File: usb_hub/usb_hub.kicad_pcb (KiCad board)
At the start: 2 copper layers, 100 x 23 mm, 120 parts, among them P1 CONN_01X02, U1 TPS2044B, U10 USB_A_FEMALE, U11 SN75240, U12 SN75240, U13 USB_A_FEMALE, U14 USB_A_FEMALE, U15 USB_A_FEMALE, U16 USB_A_FEMALE, U2 TPS2044B, U3 TUSB2077A, U4 TPS76333, U5 USB_A_MALE, U6 SN75240, U7 SN75240, U8 USB_A_FEMALE, U9 USB_A_FEMALE, X1 6 MHz

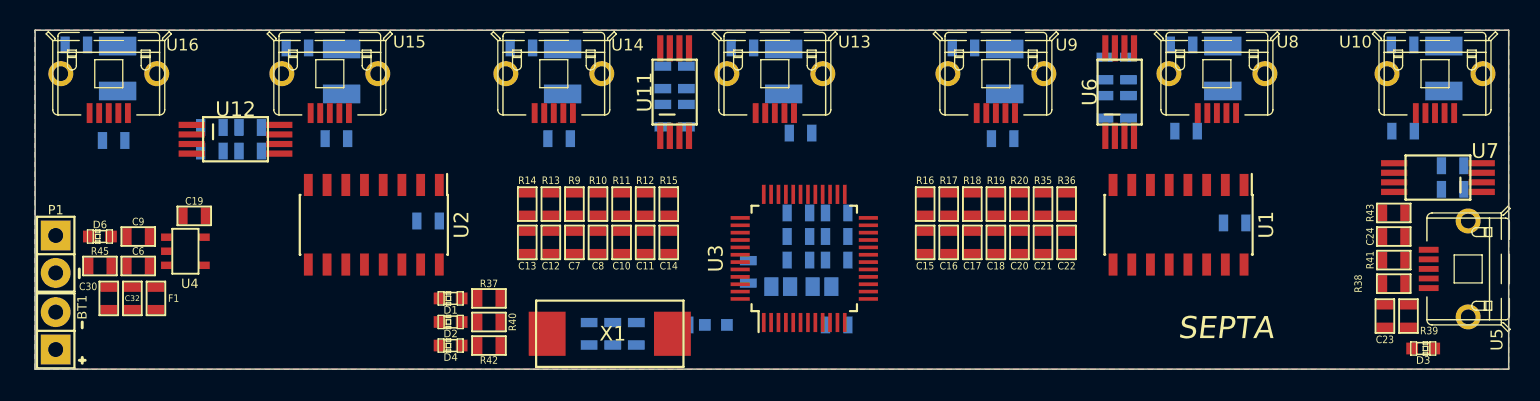
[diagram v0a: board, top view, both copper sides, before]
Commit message: finished routing. need to check bom and trace widths and pos file
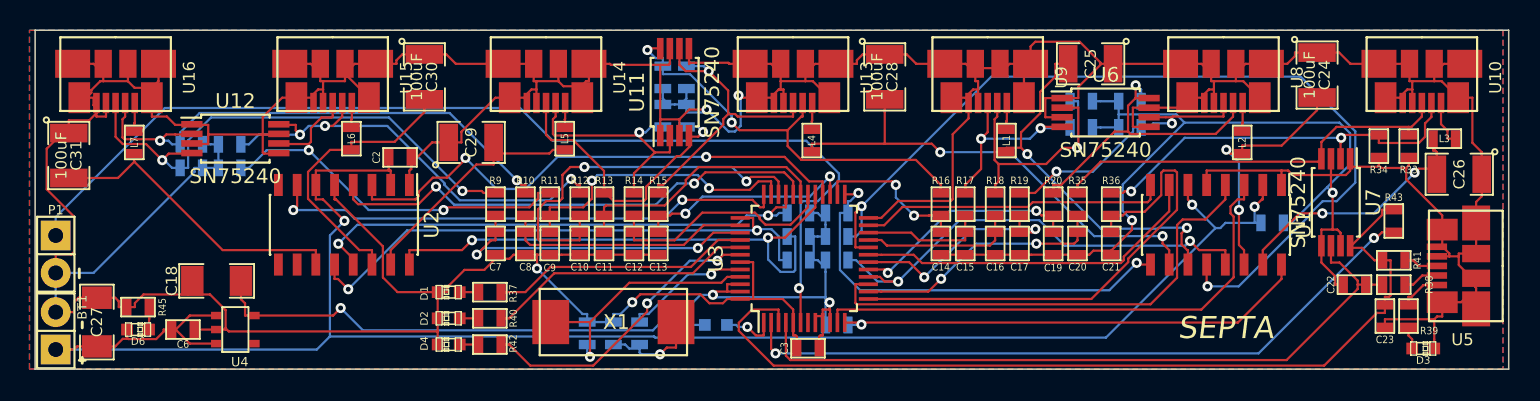
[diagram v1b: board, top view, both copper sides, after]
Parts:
- removed C32: 4.7uF, SMD_Packages:SMD-0603
- removed C33, C34, C35, C36: 100uF, SMD_Packages:SMD-1210
- removed C37, C38, C39, C40: .1uF, SMD_Packages:SMD-0603
- removed F1: FUSE, SMD_Packages:SMD-0603
- removed JP1, JP2: JUMPER, Connect:GS2
- C18: value 22pF -> 10uF; footprint SMD_Packages:SMD-0603 -> SMD_Packages:SMD-1206
- C19: value 4.7uF -> 22pF
- C2, C25, C26, C29, C3, L1, L2, L3, L4, L5, L6, L7, R33, R34: moved to F.Cu
- C24: value 22pF -> 100uF; footprint SMD_Packages:SMD-0603 -> SMD_Packages:SMD-1210
- C27: value .1uF -> 10uF; footprint SMD_Packages:SMD-0603 -> SMD_Packages:SMD-1206; moved to F.Cu
- C28, C31: value .1uF -> 100uF; footprint SMD_Packages:SMD-0603 -> SMD_Packages:SMD-1210; moved to F.Cu
- C30: value .1uF -> 100uF; footprint SMD_Packages:SMD-0603 -> SMD_Packages:SMD-1210
- C6: value 4.7uF -> 1uF
- C9: value .1uF -> 22pF
- D1, D2, D4, D6: value LED(G) -> LED
- R10, R11, R12, R13, R14, R15, R16, R17, R18, R19, R20, R35, R36, R38, R41, R9: value 27 -> 30
- R37, R39, R40, R42, R44, R45: value 510 -> 1k
- U10, U13, U14, U15, U16, U8, U9: value USB_A_FEMALE -> USB_MICRO_OUT; footprint ab2_usb:AB2_USB_MICRO_SMD -> apro_lib:MICRO_USB
- U11, U12, U6, U7: footprint usb_hub:TSSOP8 -> Housings_SSOP:TSSOP-8_4.4x3mm_Pitch0.65mm
- U5: footprint ab2_usb:AB2_USB_MICRO_SMD -> apro_lib:MICRO_USB
- moved C31 90.8 mm to (137.3, 87.5), turned to 270 degrees
- moved C27 76.0 mm to (139.2, 98.8), turned to 90 degrees
- moved C29 66.2 mm to (164.6, 86.6), turned to 0 degrees
- moved C19 58.3 mm to (204.1, 93.5), turned to 270 degrees
- moved C18 52.9 mm to (147.3, 96.0), turned to 180 degrees
- moved C26 31.6 mm to (231.6, 88.8), turned to 180 degrees
- moved C9 27.9 mm to (169.9, 93.5), turned to 270 degrees
- moved C30 26.2 mm to (161.4, 82.2), turned to 270 degrees
- moved C22 19.7 mm to (224.5, 96.3), turned to 180 degrees
- moved C14 18.5 mm to (196.5, 93.5)
- moved C24 12.1 mm to (222.0, 82.0), turned to 270 degrees
- moved C25 8.98 mm to (206.6, 81.3), turned to 180 degrees
- moved C13 8.89 mm to (177.3, 93.5)
- moved R14 7.24 mm to (175.6, 90.8)
- moved U7 7.13 mm to (223.3, 90.7), turned to 270 degrees
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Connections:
- BT1 pad 1: Net-(BT1-Pad1) -> VCC
- C18 pad 1: Net-(C18-Pad1) -> 3.3V
- C19 pad 1: 3.3V -> Net-(C19-Pad1)
- C22 pad 1: Net-(C22-Pad1) -> DM0
- C23 pad 1: DM0 -> DP0
- C24 pad 1: DP0 -> GND
- C24 pad 2: GND -> OUT2
- C25 pad 2: OUT2 -> OUT3
- C26 pad 2: OUT3 -> OUT1
- C27 pad 1: GND -> VCC
- C27 pad 2: OUT2 -> GND
- C28 pad 2: OUT3 -> OUT4
- C29 pad 2: OUT1 -> OUT5
- C30 pad 1: Net-(BT1-Pad1) -> GND
- C30 pad 2: GND -> OUT6
- C31 pad 2: OUT1 -> OUT7
- C9 pad 1: VCC -> Net-(C9-Pad1)
- R11 pad 1: Net-(C10-Pad1) -> Net-(C9-Pad1)
- R12 pad 1: Net-(C11-Pad1) -> Net-(C10-Pad1)
- R13 pad 1: Net-(C12-Pad1) -> Net-(C11-Pad1)
- R14 pad 1: Net-(C13-Pad1) -> Net-(C12-Pad1)
- R15 pad 1: Net-(C14-Pad1) -> Net-(C13-Pad1)
- R16 pad 1: Net-(C15-Pad1) -> Net-(C14-Pad1)
- R17 pad 1: Net-(C16-Pad1) -> Net-(C15-Pad1)
- R18 pad 1: Net-(C17-Pad1) -> Net-(C16-Pad1)
- R19 pad 1: Net-(C18-Pad1) -> Net-(C17-Pad1)
- R20 pad 1: Net-(C20-Pad1) -> Net-(C19-Pad1)
- R35 pad 1: Net-(C21-Pad1) -> Net-(C20-Pad1)
- R36 pad 1: Net-(C22-Pad1) -> Net-(C21-Pad1)
- R38 pad 1: Net-(R38-Pad1) -> DM0
- R38 pad 2: DM0 -> Net-(R38-Pad2)
- R41 pad 1: Net-(R41-Pad1) -> DP0
- R41 pad 2: DP0 -> Net-(R41-Pad2)
- R43 pad 1: DP0 -> DP0PUR
- R43 pad 2: DP0PUR -> DP0
- U3 pad 13: Net-(C22-Pad1) -> Net-(C21-Pad1)
- U3 pad 14: Net-(C21-Pad1) -> Net-(C20-Pad1)
- U3 pad 17: Net-(C20-Pad1) -> Net-(C19-Pad1)
- U3 pad 18: Net-(C18-Pad1) -> Net-(C17-Pad1)
- U3 pad 21: Net-(C17-Pad1) -> Net-(C16-Pad1)
- U3 pad 22: Net-(C16-Pad1) -> Net-(C15-Pad1)
- U3 pad 26: Net-(C15-Pad1) -> Net-(C14-Pad1)
- U3 pad 27: Net-(C14-Pad1) -> Net-(C13-Pad1)
- U3 pad 30: Net-(C13-Pad1) -> Net-(C12-Pad1)
- U3 pad 31: Net-(C12-Pad1) -> Net-(C11-Pad1)
- U3 pad 34: Net-(C11-Pad1) -> Net-(C10-Pad1)
- U3 pad 35: Net-(C10-Pad1) -> Net-(C9-Pad1)
- U3 pad 8: Net-(JP1-Pad2) -> 3.3V
- U5 pad 2: Net-(R38-Pad1) -> Net-(R38-Pad2)
- U5 pad 3: Net-(R41-Pad1) -> Net-(R41-Pad2)
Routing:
- net GND: track 0.00 -> 481.1 mm, vias 0 -> 6
- net VCC: track 0.00 -> 127.5 mm, vias 0 -> 3
- net RST: track 0.00 -> 71.2 mm, vias 0 -> 1
- net 3.3V: track 0.00 -> 64.3 mm, vias 0 -> 3
- net OC3: track 0.00 -> 63.3 mm, vias 0 -> 2
- net DP0: track 0.00 -> 62.1 mm
- net DM0: track 0.00 -> 48.9 mm
- net DP0PUR: track 0.00 -> 47.6 mm, vias 0 -> 2
- net OC7: track 0.00 -> 37.3 mm, vias 0 -> 2
- net OC5: track 0.00 -> 37.2 mm, vias 0 -> 2
- net PWRON5: track 0.00 -> 36.3 mm, vias 0 -> 2
- net DM7: track 0.00 -> 36.2 mm, vias 0 -> 2
- net DP7: track 0.00 -> 35.8 mm, vias 0 -> 2
- net PWRON1: track 0.00 -> 35.7 mm
- net PWRON7: track 0.00 -> 35.6 mm, vias 0 -> 2
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- added copper zone on B.Cu, net (none)
- added copper zone on F.Cu, net (none)
- removed copper zone on B.Cu, net GND
- removed copper zone on F.Cu, net GND
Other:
- net class Default: via_dia 0.7366 -> 0.6858; via_drill 0.381 -> 0.3302
